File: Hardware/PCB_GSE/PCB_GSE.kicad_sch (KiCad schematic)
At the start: 38 parts, among them J1 Conn_01x06_Pin, U1 STM32F103CBT6

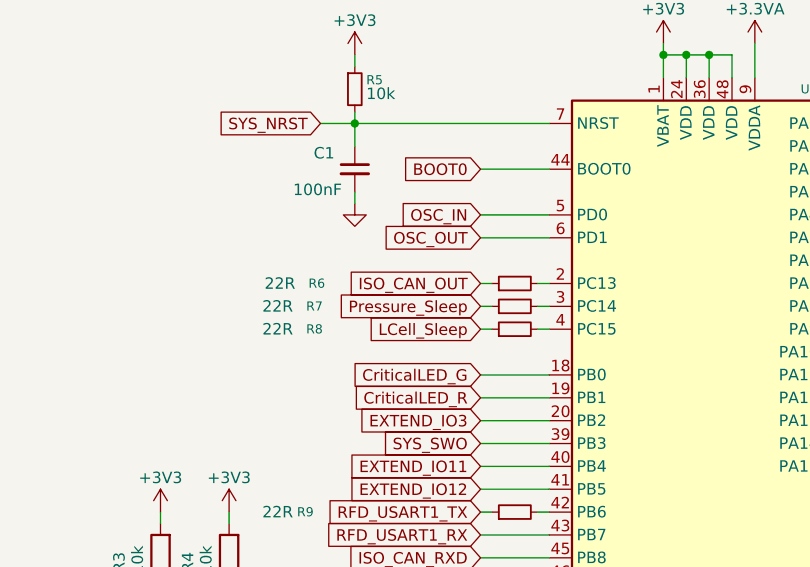
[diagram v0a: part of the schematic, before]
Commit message: wip : routing local circuits and power planes
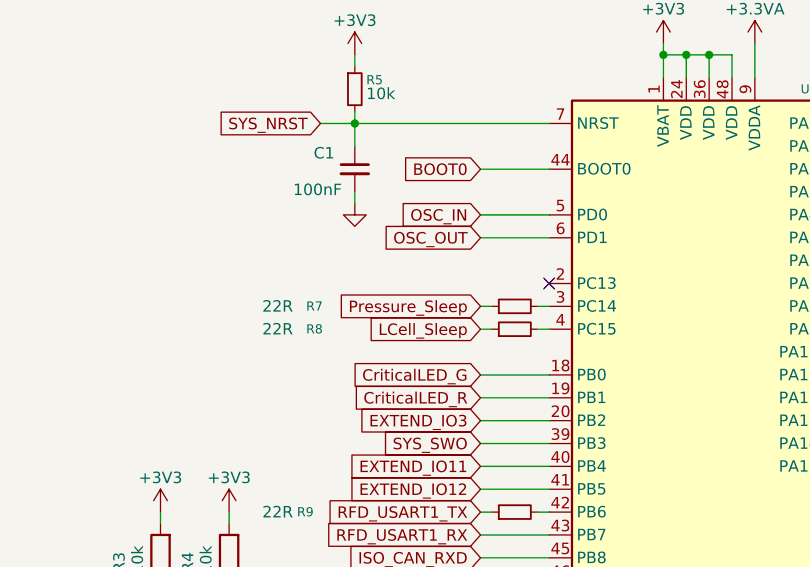
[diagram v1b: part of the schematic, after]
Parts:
- removed R6: 22R, Resistor_SMD:R_0603_1608Metric, symbol Device:R_Small
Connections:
- no-connect marks 0 -> 1
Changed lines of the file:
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@@
 		(color 0 0 0 0)
 	)
+	(no_connect
+		(at 130.81 68.58)
+	)
 	(wire
 		(pts
@@
 	(wire
 		(pts
-			(xy 123.19 68.58) (xy 124.46 68.58)
-		)
-		(stroke
-			(width 0)
-			(type default)
-		)
-	)
-	(wire
-		(pts
 			(xy 151.13 43.18) (xy 148.59 43.18)
 		)
@@
 	(wire
 		(pts
-			(xy 129.54 68.58) (xy 130.81 68.58)
-		)
-		(stroke
-			(width 0)
-			(type default)
-		)
-	)
-	(wire
-		(pts
 			(xy 148.59 43.18) (xy 146.05 43.18)
 		)
@@
 		)
 	)
-	(global_label "ISO_CAN_OUT"
-		(shape input)
-		(at 123.19 68.58 180)
-		(fields_autoplaced yes)
-		(effects
-			(font
-				(size 1.27 1.27)
-			)
-			(justify right)
-		)
-		(property "Intersheetrefs" "${INTERSHEET_REFS}"
-			(at 107.8071 68.58 0)
-			(effects
-				(font
-					(size 1.27 1.27)
-				)
-				(justify right)
-				(hide yes)
-			)
-		)
-	)
 	(global_label "Pressure_Sleep"
 		(shape input)
@@
 					(unit 1)
 				)
-			)
-		)
-	)
-	(symbol
-		(lib_id "Device:R_Small")
-		(at 127 68.58 90)
-		(unit 1)
-		(exclude_from_sim no)
-		(in_bom yes)
-		(on_board yes)
-		(dnp no)
-		(property "Reference" "R6"
-			(at 105.918 68.58 90)
-			(effects
-				(font
-					(size 1.016 1.016)
-				)
-				(justify left)
-			)
-		)
-		(property "Value" "22R"
-			(at 102.616 68.58 90)
-			(effects
-				(font
-					(size 1.27 1.27)
-				)
-				(justify left)
-			)
-		)
-		(property "Footprint" "Resistor_SMD:R_0603_1608Metric"
-			(at 127 68.58 0)
-			(effects
-				(font
-					(size 1.27 1.27)
-				)
-				(hide yes)
-			)
-		)
-		(property "Datasheet" "https://www.digikey.ca/en/products/detail/rohm-semiconductor/ESR03EZPJ220/1983463"
-			(at 127 68.58 0)
-			(effects
-				(font
-					(size 1.27 1.27)
-				)
-				(hide yes)
-			)
-		)
-		(property "Description" "Resistor, small symbol"
-			(at 127 68.58 0)
-			(effects
-				(font
-					(size 1.27 1.27)
-				)
-				(hide yes)
-			)
-		)
-		(property "DigiKey_Part_Number" "RHM22DCT-ND"
-			(at 127 68.58 90)
-			(effects
-				(font
-					(size 1.27 1.27)
-				)
-				(hide yes)
-			)
-		)
-		(property "Manufacturer_Part_Number" "ESR03EZPJ220"
-			(at 127 68.58 90)
-			(effects
-				(font
-					(size 1.27 1.27)
-				)
-				(hide yes)
-			)
-		)
-		(pin "1"
-		)
-		(pin "2"
-		)
-		(instances
-			(project "PCB_GSE"
-				(path "/a63f9ed4-21e4-42d0-8bfc-f96143f84d4d"
-					(reference "R6")
-					(unit 1)
-				)
